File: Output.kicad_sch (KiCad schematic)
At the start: 8 parts, among them J20 Output, Q4 SISA88DN or similar

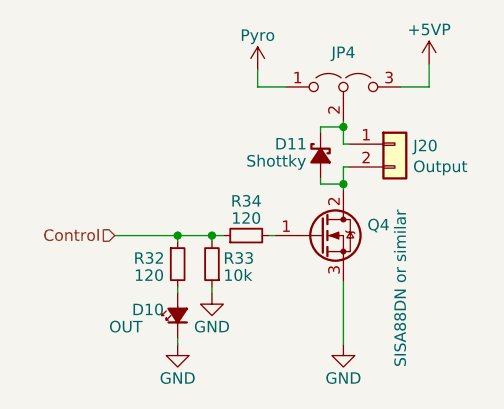
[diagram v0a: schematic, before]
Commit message: Revert "PMU V3 "ready to order?""
This reverts commit e5aaef69110c3557dfda333950fee24891806424.
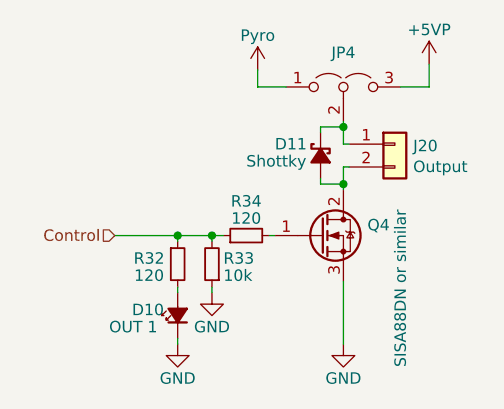
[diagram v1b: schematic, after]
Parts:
- D10: value OUT -> OUT 1
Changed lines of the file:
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@@
     (effects (font (size 1.27 1.27)) (justify right))
   )
-  (symbol (lib_id "power:GND") (at 151.765 90.805 0) (unit 1)
+  (symbol (lib_id "power:GND") (at 151.765 90.805 0)
     (in_bom yes) (on_board yes)
     (property "Reference" "#PWR083" (id 0) (at 151.765 97.155 0)
@@
     (pin "1")
   )
-  (symbol (lib_id "Jumper:Jumper_3_Open") (at 151.765 62.23 0) (unit 1)
+  (symbol (lib_id "Jumper:Jumper_3_Open") (at 151.765 62.23 0)
     (in_bom yes) (on_board yes) (fields_autoplaced)
     (property "Reference" "JP4" (id 0) (at 151.765 58.42 0))
@@
     (pin "3")
   )
-  (symbol (lib_id "Device:Q_NMOS_GDS") (at 149.225 78.74 0) (unit 1)
+  (symbol (lib_id "Device:Q_NMOS_GDS") (at 149.225 78.74 0)
     (in_bom yes) (on_board yes)
     (property "Reference" "Q4" (id 0) (at 154.432 77.5716 0)
@@
     (pin "3")
   )
-  (symbol (lib_id "Device:D_Schottky_Small_Filled") (at 149.225 69.85 90) (mirror x) (unit 1)
+  (symbol (lib_id "Device:D_Schottky_Small_Filled") (at 149.225 69.85 90) (mirror x)
     (in_bom yes) (on_board yes)
     (property "Reference" "D11" (id 0) (at 144.145 68.58 90)
@@
     (pin "2")
   )
-  (symbol (lib_id "Device:R_Small") (at 133.35 81.915 0) (unit 1)
+  (symbol (lib_id "Device:R_Small") (at 133.35 81.915 0)
     (in_bom yes) (on_board yes)
     (property "Reference" "R32" (id 0) (at 130.175 81.28 0))
@@
     (pin "2")
   )
-  (symbol (lib_id "Connector_Generic:Conn_01x02") (at 157.48 68.58 0) (unit 1)
+  (symbol (lib_id "Connector_Generic:Conn_01x02") (at 157.48 68.58 0)
     (in_bom yes) (on_board yes)
     (property "Reference" "J20" (id 0) (at 159.512 68.7832 0)
@@
     (pin "2")
   )
-  (symbol (lib_id "power:GND") (at 133.35 90.805 0) (unit 1)
+  (symbol (lib_id "power:GND") (at 133.35 90.805 0)
     (in_bom yes) (on_board yes)
     (property "Reference" "#PWR080" (id 0) (at 133.35 97.155 0)
@@
     (pin "1")
   )
-  (symbol (lib_id "Device:R_Small") (at 137.16 81.915 180) (unit 1)
+  (symbol (lib_id "Device:R_Small") (at 137.16 81.915 180)
     (in_bom yes) (on_board yes)
     (property "Reference" "R33" (id 0) (at 138.43 81.28 0)
@@
     (pin "2")
   )
-  (symbol (lib_id "power:GND") (at 137.16 85.09 0) (unit 1)
+  (symbol (lib_id "power:GND") (at 137.16 85.09 0)
     (in_bom yes) (on_board yes)
     (property "Reference" "#PWR081" (id 0) (at 137.16 91.44 0)
@@
     (pin "1")
   )
-  (symbol (lib_id "Device:LED_Small_Filled") (at 133.35 87.63 90) (unit 1)
+  (symbol (lib_id "Device:LED_Small_Filled") (at 133.35 87.63 90)
     (in_bom yes) (on_board yes)
     (property "Reference" "D10" (id 0) (at 128.27 86.995 90)
       (effects (font (size 1.27 1.27)) (justify right))
     )
-    (property "Value" "OUT" (id 1) (at 125.73 88.9 90)
+    (property "Value" "OUT 1" (id 1) (at 125.73 88.9 90)
       (effects (font (size 1.27 1.27)) (justify right))
     )
@@
     (pin "2")
   )
-  (symbol (lib_id "power:+5VP") (at 161.29 59.69 0) (unit 1)
+  (symbol (lib_id "power:+5VP") (at 161.29 59.69 0)
     (in_bom yes) (on_board yes)
     (property "Reference" "#PWR084" (id 0) (at 161.29 63.5 0)
@@
     (pin "1")
   )
-  (symbol (lib_id "Device:R_Small") (at 140.97 78.74 90) (unit 1)
+  (symbol (lib_id "Device:R_Small") (at 140.97 78.74 90)
     (in_bom yes) (on_board yes)
     (property "Reference" "R34" (id 0) (at 140.97 74.93 90))
@@
     (pin "2")
   )
-  (symbol (lib_id "TXV_Library_Symbols:Pyro") (at 142.24 60.325 0) (unit 1)
+  (symbol (lib_id "TXV_Library_Symbols:Pyro") (at 142.24 60.325 0)
     (in_bom yes) (on_board yes)
     (property "Reference" "#PWR082" (id 0) (at 142.24 64.135 0)

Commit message: PMU V3 "ready to order?"
ready to validate changes
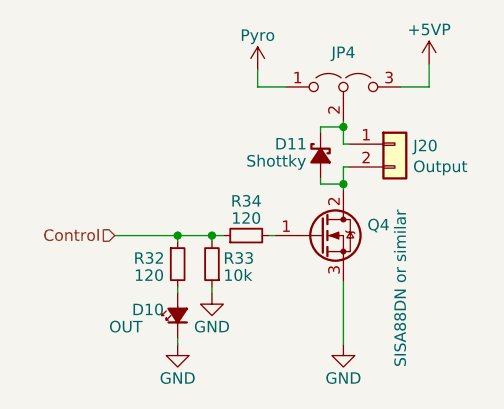
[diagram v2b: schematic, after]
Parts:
- D10: value OUT 1 -> OUT
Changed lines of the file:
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@@
     (effects (font (size 1.27 1.27)) (justify right))
   )
-  (symbol (lib_id "power:GND") (at 151.765 90.805 0)
+  (symbol (lib_id "power:GND") (at 151.765 90.805 0) (unit 1)
     (in_bom yes) (on_board yes)
     (property "Reference" "#PWR083" (id 0) (at 151.765 97.155 0)
@@
     (pin "1")
   )
-  (symbol (lib_id "Jumper:Jumper_3_Open") (at 151.765 62.23 0)
+  (symbol (lib_id "Jumper:Jumper_3_Open") (at 151.765 62.23 0) (unit 1)
     (in_bom yes) (on_board yes) (fields_autoplaced)
     (property "Reference" "JP4" (id 0) (at 151.765 58.42 0))
@@
     (pin "3")
   )
-  (symbol (lib_id "Device:Q_NMOS_GDS") (at 149.225 78.74 0)
+  (symbol (lib_id "Device:Q_NMOS_GDS") (at 149.225 78.74 0) (unit 1)
     (in_bom yes) (on_board yes)
     (property "Reference" "Q4" (id 0) (at 154.432 77.5716 0)
@@
     (pin "3")
   )
-  (symbol (lib_id "Device:D_Schottky_Small_Filled") (at 149.225 69.85 90) (mirror x)
+  (symbol (lib_id "Device:D_Schottky_Small_Filled") (at 149.225 69.85 90) (mirror x) (unit 1)
     (in_bom yes) (on_board yes)
     (property "Reference" "D11" (id 0) (at 144.145 68.58 90)
@@
     (pin "2")
   )
-  (symbol (lib_id "Device:R_Small") (at 133.35 81.915 0)
+  (symbol (lib_id "Device:R_Small") (at 133.35 81.915 0) (unit 1)
     (in_bom yes) (on_board yes)
     (property "Reference" "R32" (id 0) (at 130.175 81.28 0))
@@
     (pin "2")
   )
-  (symbol (lib_id "Connector_Generic:Conn_01x02") (at 157.48 68.58 0)
+  (symbol (lib_id "Connector_Generic:Conn_01x02") (at 157.48 68.58 0) (unit 1)
     (in_bom yes) (on_board yes)
     (property "Reference" "J20" (id 0) (at 159.512 68.7832 0)
@@
     (pin "2")
   )
-  (symbol (lib_id "power:GND") (at 133.35 90.805 0)
+  (symbol (lib_id "power:GND") (at 133.35 90.805 0) (unit 1)
     (in_bom yes) (on_board yes)
     (property "Reference" "#PWR080" (id 0) (at 133.35 97.155 0)
@@
     (pin "1")
   )
-  (symbol (lib_id "Device:R_Small") (at 137.16 81.915 180)
+  (symbol (lib_id "Device:R_Small") (at 137.16 81.915 180) (unit 1)
     (in_bom yes) (on_board yes)
     (property "Reference" "R33" (id 0) (at 138.43 81.28 0)
@@
     (pin "2")
   )
-  (symbol (lib_id "power:GND") (at 137.16 85.09 0)
+  (symbol (lib_id "power:GND") (at 137.16 85.09 0) (unit 1)
     (in_bom yes) (on_board yes)
     (property "Reference" "#PWR081" (id 0) (at 137.16 91.44 0)
@@
     (pin "1")
   )
-  (symbol (lib_id "Device:LED_Small_Filled") (at 133.35 87.63 90)
+  (symbol (lib_id "Device:LED_Small_Filled") (at 133.35 87.63 90) (unit 1)
     (in_bom yes) (on_board yes)
     (property "Reference" "D10" (id 0) (at 128.27 86.995 90)
       (effects (font (size 1.27 1.27)) (justify right))
     )
-    (property "Value" "OUT 1" (id 1) (at 125.73 88.9 90)
+    (property "Value" "OUT" (id 1) (at 125.73 88.9 90)
       (effects (font (size 1.27 1.27)) (justify right))
     )
@@
     (pin "2")
   )
-  (symbol (lib_id "power:+5VP") (at 161.29 59.69 0)
+  (symbol (lib_id "power:+5VP") (at 161.29 59.69 0) (unit 1)
     (in_bom yes) (on_board yes)
     (property "Reference" "#PWR084" (id 0) (at 161.29 63.5 0)
@@
     (pin "1")
   )
-  (symbol (lib_id "Device:R_Small") (at 140.97 78.74 90)
+  (symbol (lib_id "Device:R_Small") (at 140.97 78.74 90) (unit 1)
     (in_bom yes) (on_board yes)
     (property "Reference" "R34" (id 0) (at 140.97 74.93 90))
@@
     (pin "2")
   )
-  (symbol (lib_id "TXV_Library_Symbols:Pyro") (at 142.24 60.325 0)
+  (symbol (lib_id "TXV_Library_Symbols:Pyro") (at 142.24 60.325 0) (unit 1)
     (in_bom yes) (on_board yes)
     (property "Reference" "#PWR082" (id 0) (at 142.24 64.135 0)
